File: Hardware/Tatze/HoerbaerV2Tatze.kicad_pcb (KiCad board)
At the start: 2 copper layers, 80 x 84 mm, 15 parts, among them J8 PAW_A, J9 PAW_A, SW1 SW_Push, SW2 SW_Push, SW3 SW_Push, SW4 SW_Push, SW5 SW_Push

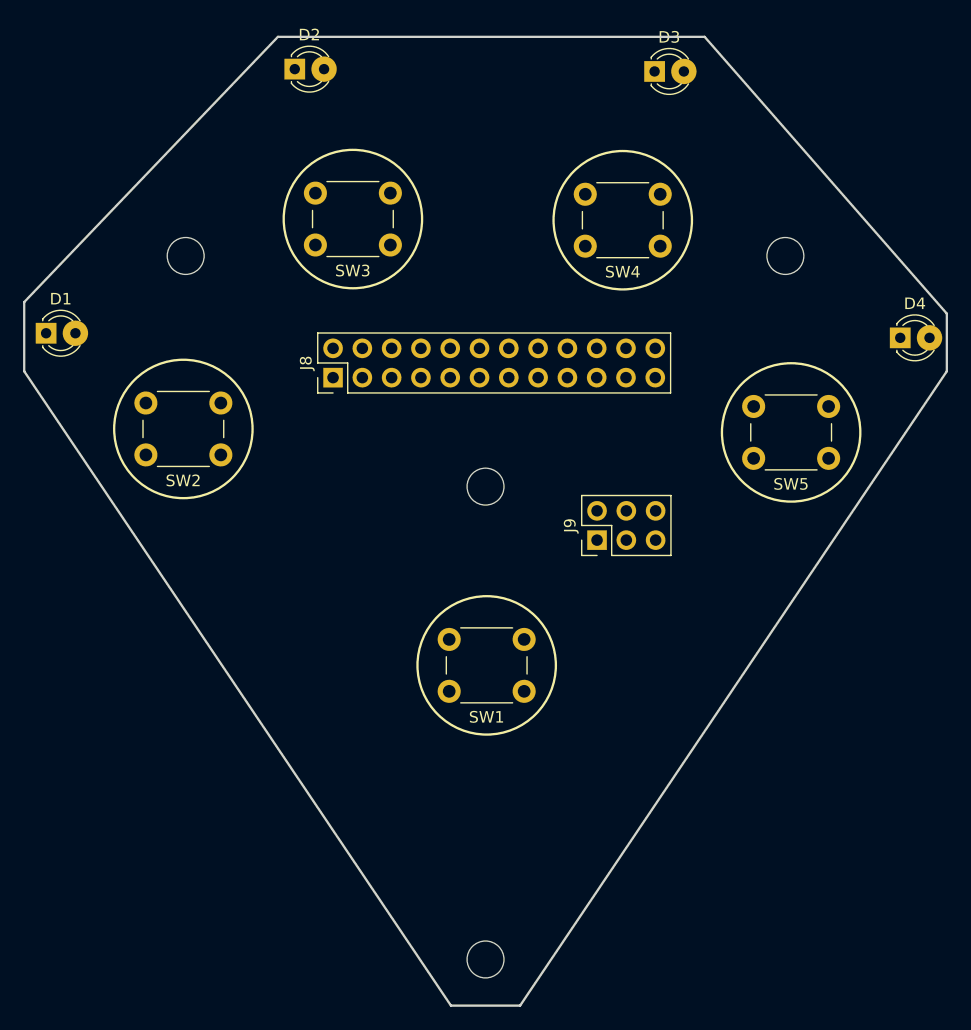
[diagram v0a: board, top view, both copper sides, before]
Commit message: Paw
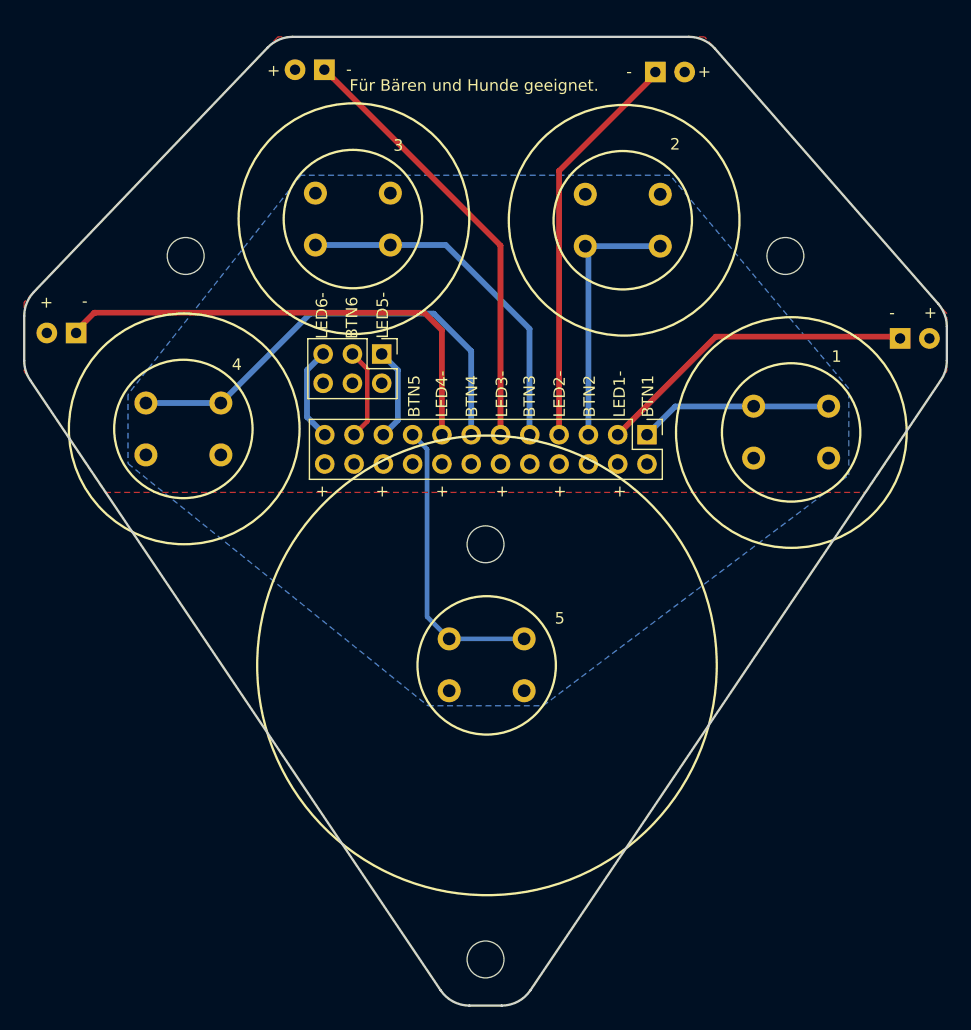
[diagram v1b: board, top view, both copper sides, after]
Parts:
- removed the MH1 at (74.9, 63.5)
- added MH2: MountingHole, MountingHole:MountingHole_3.2mm_M3, F.Cu at (74.9, 68.5)
- D1: renamed from D4; moved to B.Cu
- D2: renamed from D3; moved to B.Cu
- D3: renamed from D2; moved to B.Cu
- D4: renamed from D1; moved to B.Cu
- SW1: renamed from SW5; moved to B.Cu
- SW2: renamed from SW4; moved to B.Cu
- SW3: moved to B.Cu
- SW4: renamed from SW2; moved to B.Cu
- SW5: renamed from SW1; moved to B.Cu
- moved J8 27.7 mm to (88.9, 59.0), turned to -90 degrees
- moved J9 24.7 mm to (65.9, 52.0), turned to -90 degrees
- moved SW3 6.50 mm to (66.7, 38.0), turned to 180 degrees
- moved SW2 6.50 mm to (90.0, 38.1), turned to 180 degrees
- moved SW4 4.50 mm to (45.5, 60.8)
- moved SW1 4.48 mm to (98.2, 61.0)
- moved SW5 4.45 mm to (71.8, 81.2)
- moved D4 2.60 mm to (39.4, 50.2), turned to 180 degrees
- moved D3 2.57 mm to (60.9, 27.4), turned to 180 degrees
- moved D2 0.08 mm to (89.6, 27.6)
- moved D1 0.05 mm to (110.8, 50.6)
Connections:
- D1 pad 1: /PAW_A_D4 -> /PAW_A_D1
- D2 pad 1: /PAW_A_D3 -> /PAW_A_D2
- D3 pad 1: /PAW_A_D2 -> /PAW_A_D3
- D4 pad 1: /PAW_A_D1 -> /PAW_A_D4
- SW1 pad 2: /PAW_A_B5 -> /PAW_A_B1
- SW2 pad 2: /PAW_A_B4 -> /PAW_A_B2
- SW4 pad 2: /PAW_A_B2 -> /PAW_A_B4
- SW5 pad 2: /PAW_A_B1 -> /PAW_A_B5
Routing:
- net /PAW_A_D4: track 0.00 -> 42.2 mm
- net /PAW_A_B4: track 0.00 -> 40.0 mm
- net /PAW_A_D3: track 0.00 -> 38.0 mm
- net /PAW_A_D2: track 0.00 -> 34.9 mm
- net /PAW_A_B3: track 0.00 -> 30.8 mm
- net /PAW_A_D1: track 0.00 -> 28.1 mm
- net /PAW_A_B5: track 0.00 -> 25.5 mm
- net /PAW_A_B2: track 0.00 -> 23.0 mm
- net /PAW_A_B1: track 0.00 -> 16.8 mm
- net /PAW_A_D6: track 0.00 -> 8.22 mm
- net /PAW_A_D5: track 0.00 -> 8.10 mm
- net /PAW_A_B6: track 0.00 -> 8.01 mm
- added copper zone on F.Cu, net +9V
- added copper zone on B.Cu, net GND
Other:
- outline, holes or cut-outs redrawn
- board text added: "+"
- board text added: "-"
- board text added: "1"
- board text added: "2"
- board text added: "3"
- board text added: "4"
- board text added: "5"
- board text added: "BTN1"
- board text added: "BTN2"
- board text added: "BTN3"
- board text added: "BTN4"
- board text added: "BTN5"
- board text added: "BTN6"
- board text added: "Für Bären und Hunde geeignet."
- board text added: "LED1-"
- board text added: "LED2-"
- board text added: "LED3-"
- board text added: "LED4-"
- board text added: "LED5-"
- board text added: "LED6-"
